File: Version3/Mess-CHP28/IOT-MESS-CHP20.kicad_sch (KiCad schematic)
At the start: 25 parts, among them J1 Jumper_2, J2 Jumper_2, J3 Jumper, J4 Conn_01x15_Pin, J5 Conn_01x15_Pin, J6 Jumper, J7 Jumper_2, J9 Jumper_2, K1 Crystal, U4 USB_C_Receptacle_USB2.0_16P, U5 ME6211C33M5, U6 XC6206PxxxMR

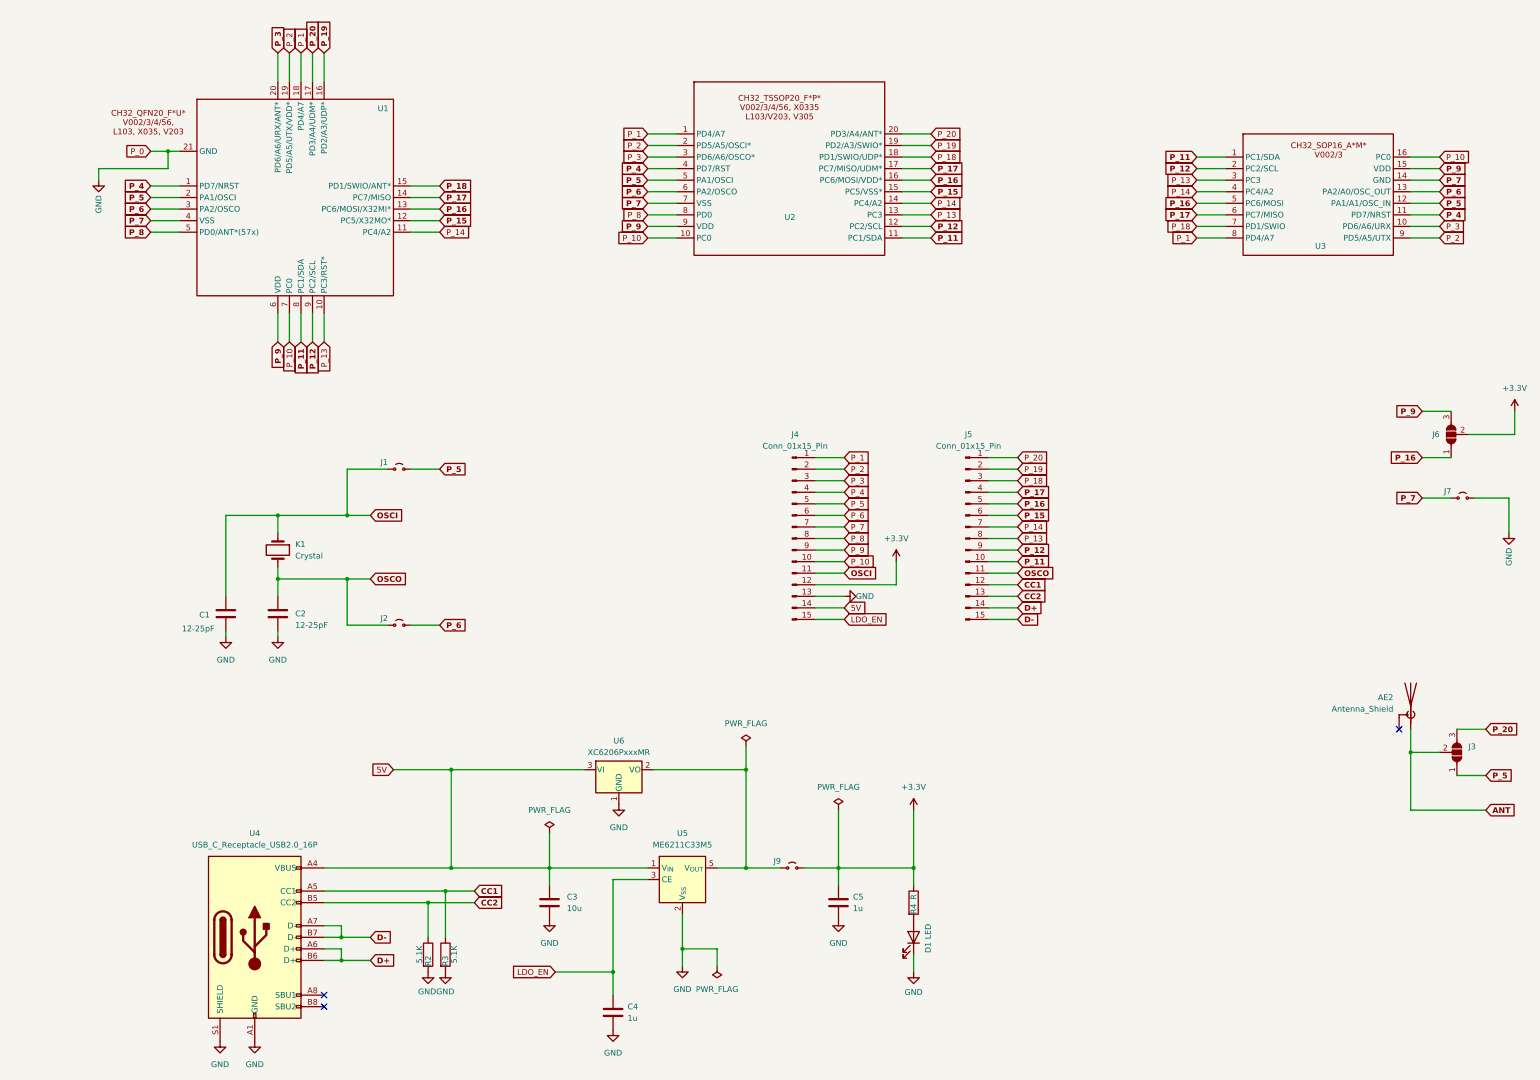
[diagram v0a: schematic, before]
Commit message: update.
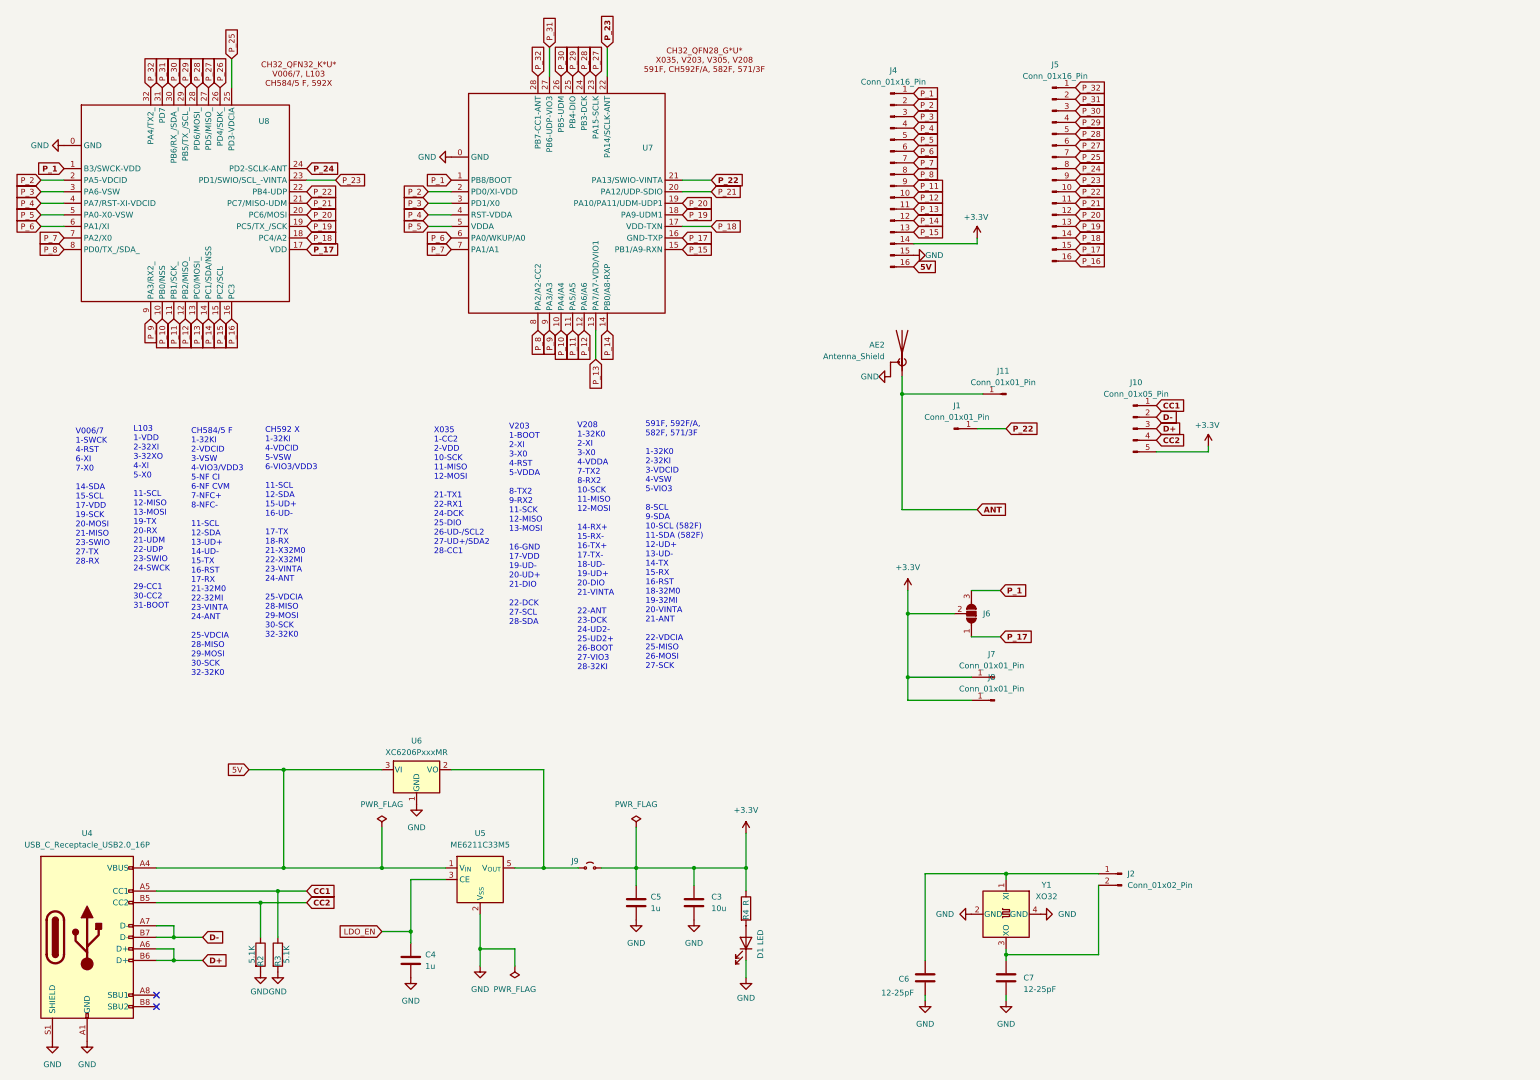
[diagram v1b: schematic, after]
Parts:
- removed C1, C2: 12-25pF, Capacitor_SMD:C_0603_1608Metric, symbol Device:C
- removed J1, J2, J7: Jumper_2, IOT-Mess-Footprints:Jumpper-triangle, symbol Jumper:Jumper_2_Small_Open
- removed J3: Jumper, IOT-Mess-Footprints:Jumper-3_P1.3mm_Open_RoundedPad1.0x1.5mm, symbol Jumper:SolderJumper_3_Open
- removed J4, J5: Conn_01x15_Pin, Connector_PinHeader_2.54mm:PinHeader_1x15_P2.54mm_Vertical, symbol Connector:Conn_01x15_Pin
- removed K1: Crystal, Crystal:Crystal_SMD_3225-4Pin_3.2x2.5mm, symbol Device:Crystal
- removed U1: ~, Package_DFN_QFN:QFN-20-1EP_3x3mm_P0.4mm_EP1.65x1.65mm_ThermalVias, symbol IOT-Mess:CH32_QFN20_F*U*
- removed U2: ~, Package_SO:TSSOP-20_4.4x6.5mm_P0.65mm, symbol IOT-Mess:CH32_TSSOP20_F*P*
- removed U3: ~, Package_SO:SOP-16_3.9x9.9mm_P1.27mm, symbol IOT-Mess:CH32_SOP16_A*M*
- added C6, C7: 12-25pF, Capacitor_SMD:C_0603_1608Metric, symbol Device:C
- added J1, J11, J7, J8: Conn_01x01_Pin, Connector_PinHeader_1.00mm:PinHeader_1x01_P1.00mm_Vertical, symbol Connector:Conn_01x01_Pin
- added J10: Conn_01x05_Pin, Connector_PinHeader_1.27mm:PinHeader_1x05_P1.27mm_Vertical, symbol Connector:Conn_01x05_Pin
- added J2: Conn_01x02_Pin, Connector_PinHeader_1.27mm:PinHeader_1x02_P1.27mm_Vertical, symbol Connector:Conn_01x02_Pin
- added J4, J5: Conn_01x16_Pin, Connector_PinHeader_2.54mm:PinHeader_1x16_P2.54mm_Vertical, symbol Connector:Conn_01x16_Pin
- added U7: ~, Package_DFN_QFN:QFN-28-1EP_4x4mm_P0.4mm_EP2.4x2.4mm_ThermalVias, symbol My_Symbol_Lib:CH32_QFN28_G*U*
- added U8: ~, Package_DFN_QFN:QFN-32-1EP_4x4mm_P0.4mm_EP2.65x2.65mm_ThermalVias, symbol My_Symbol_Lib:CH32_QFN32_K*U*
- added Y1: XO32, Oscillator:Oscillator_SMD_EuroQuartz_XO32-4Pin_3.2x2.5mm, symbol Oscillator:XO32
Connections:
- net +3.3V: now also C3.1, J10.5 (Pin_5), J4.14 (Pin_14), J7.1 (Pin_1), J8.1 (Pin_1)
- net 5V: now also J4.16 (Pin_16); no longer C3.1
- net ANT: now also J11.1 (Pin_1)
- net CC1: now also J10.1 (Pin_1)
- net CC2: now also J10.4 (Pin_4)
- net D+: now also J10.3 (Pin_3)
- net D-: now also J10.2 (Pin_2)
- net GND: now also AE2.2 (Shield), C6.2, C7.2, J4.15 (Pin_15), U7.0 (GND), U8.0 (GND), Y1.2 (GND), Y1.4 (GND)
- net P_1: now also J6.3 (B), J4.1 (Pin_1), U7.1 (PB8/BOOT), U8.1 (B3/SWCK-VDD)
- net P_10: now also U7.10 (PA4/A4), U8.10 (PB0/NSS)
- net P_11: now also J4.9 (Pin_9), U7.11 (PA5/A5), U8.11 (PB1/SCK_)
- net P_12: now also J4.10 (Pin_10), U7.12 (PA6/A6), U8.12 (PB2/MISO_)
- net P_13: now also J4.11 (Pin_11), U7.13 (PA7/A7-VDD/VIO1), U8.13 (PC0/MOSI_)
- net P_14: now also J4.12 (Pin_12), U7.14 (PB0/A8-RXP), U8.14 (PC1/SDA/NSS)
- net P_15: now also J4.13 (Pin_13), U7.15 (PB1/A9-RXN), U8.15 (PC2/SCL)
- net P_16: now also J5.16 (Pin_16), U8.16 (PC3); no longer J6.1 (A)
- net P_17: now also J6.1 (A), J5.15 (Pin_15), U7.16 (GND-TXP), U8.17 (VDD)
- net P_18: now also J5.14 (Pin_14), U7.17 (VDD-TXN), U8.18 (PC4/A2)
- net P_19: now also J5.13 (Pin_13), U7.18 (PA9-UDM1), U8.19 (PC5/TX_/SCK)
- net P_2: now also J4.2 (Pin_2), U7.2 (PD0/XI-VDD), U8.2 (PA5-VDCID)
- net P_20: now also J5.12 (Pin_12), U7.19 (PA10/PA11/UDM-UDP1), U8.20 (PC6/MOSI)
- net P_3: now also J4.3 (Pin_3), U7.3 (PD1/X0), U8.3 (PA6-VSW)
- net P_4: now also J4.4 (Pin_4), U7.4 (RST-VDDA), U8.4 (PA7/RST-XI-VDCID)
- net P_5: now also J4.5 (Pin_5), U7.5 (VDDA), U8.5 (PA0-X0-VSW)
- net P_6: now also J4.6 (Pin_6), U7.6 (PA0/WKUP/A0), U8.6 (PA1/XI)
- net P_7: now also J4.7 (Pin_7), U7.7 (PA1/A1), U8.7 (PA2/X0)
- net P_8: now also J4.8 (Pin_8), U7.8 (PA2/A2-CC2), U8.8 (PD0/TX_/SDA_)
- net P_9: now also U7.9 (PA3/A3), U8.9 (PA3/RX2_); no longer J6.3 (B)
- new net: C6.1, J2.1 (Pin_1), Y1.1 (XI)
- new net: C7.1, J2.2 (Pin_2), Y1.3 (XO)
- new net P_21: J5.11 (Pin_11), U7.20 (PA12/UDP-SDIO), U8.21 (PC7/MISO-UDM)
- new net P_22: J1.1 (Pin_1), J5.10 (Pin_10), U7.21 (PA13/SWIO-VINTA), U8.22 (PB4-UDP)
- new net P_23: J5.9 (Pin_9), U7.22 (PA14/SCLK-ANT), U8.23 (PD1/SWIO/SCL_-VINTA)
- new net P_24: J5.8 (Pin_8), U8.24 (PD2-SCLK-ANT)
- new net P_25: J5.7 (Pin_7), U8.25 (PD3-VDCIA)
- new net P_26: U8.26 (PD4/SDK_)
- new net P_27: J5.6 (Pin_6), U7.23 (PA15-SCLK), U8.27 (PD5/MISO_)
- new net P_28: J5.5 (Pin_5), U7.24 (PB3-DCK), U8.28 (PD6/MOSI_)
- new net P_29: J5.4 (Pin_4), U7.25 (PB4-DIO), U8.29 (PB5/TX_/SCL_)
- new net P_30: J5.3 (Pin_3), U7.26 (PB5-UDM), U8.30 (PB6/RX_/SDA_)
- new net P_31: J5.2 (Pin_2), U7.27 (PB6-UDP-VIO3), U8.31 (PD7)
- new net P_32: J5.1 (Pin_1), U7.28 (PB7-CC1-ANT), U8.32 (PA4/TX2_)
- no-connect marks 3 -> 2
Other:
- note added: "591F, 592F/A, 582F, 571/3F 1-32K0 2-32KI 3-VDCID 4-VSW 5-VIO3 8-SCL 9-SDA 10-SCL (582F) 11-SDA (582F) 12-UD+ 13-UD- 14-TX 15-RX 16-RST 18-32M0 19-32MI 20-VINTA 21-ANT 22-VDCIA 25-MISO 26-MOSI 27-SCK"
- note added: "CH584/5 F 1-32KI 2-VDCID 3-VSW 4-VIO3/VDD3 5-NF CI 6-NF CVM 7-NFC+ 8-NFC- 11-SCL 12-SDA 13-UD+ 14-UD- 15-TX 16-RST 17-RX 21-32M0 22-32MI 23-VINTA 24-ANT 25-VDCIA 28-MISO 29-MOSI 30-SCK 32-32K0"
- note added: "CH592 X 1-32KI 4-VDCID 5-VSW 6-VIO3/VDD3 11-SCL 12-SDA 15-UD+ 16-UD- 17-TX 18-RX 21-X32M0 22-X32MI 23-VINTA 24-ANT 25-VDCIA 28-MISO 29-MOSI 30-SCK 32-32K0"
- note added: "L103 1-VDD 2-32XI 3-32XO 4-XI 5-X0 11-SCL 12-MISO 13-MOSI 19-TX 20-RX 21-UDM 22-UDP 23-SWIO 24-SWCK 29-CC1 30-CC2 31-BOOT"
- note added: "V006/7 1-SWCK 4-RST 6-XI 7-X0 14-SDA 15-SCL 17-VDD 19-SCK 20-MOSI 21-MISO 23-SWIO 27-TX 28-RX"
- note added: "V203 1-BOOT 2-XI 3-X0 4-RST 5-VDDA 8-TX2 9-RX2 11-SCK 12-MISO 13-MOSI 16-GND 17-VDD 19-UD- 20-UD+ 21-DIO 22-DCK 27-SCL 28-SDA"
- note added: "V208 1-32K0 2-XI 3-X0 4-VDDA 7-TX2 8-RX2 10-SCK 11-MISO 12-MOSI 14-RX+ 15-RX- 16-TX+ 17-TX- 18-UD- 19-UD+ 20-DIO 21-VINTA 22-ANT 23-DCK 24-UD2- 25-UD2+ 26-BOOT 27-VIO3 28-32KI"
- note added: "X035 1-CC2 2-VDD 10-SCK 11-MISO 12-MOSI 21-TX1 22-RX1 24-DCK 25-DIO 26-UD-/SCL2 27-UD+/SDA2 28-CC1"
- moved on the sheet: AE2, C3, C4, C5, D1, J6, J9, R2, R3, R4, U4, U5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
